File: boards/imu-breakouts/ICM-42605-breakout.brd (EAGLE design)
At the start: 15.2 x 12.7 mm, 5 parts, among them U3 ICM-42605

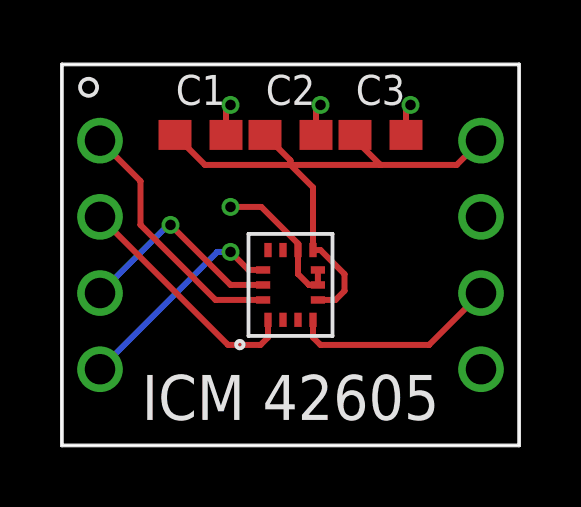
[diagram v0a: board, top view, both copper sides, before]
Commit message: IMU done
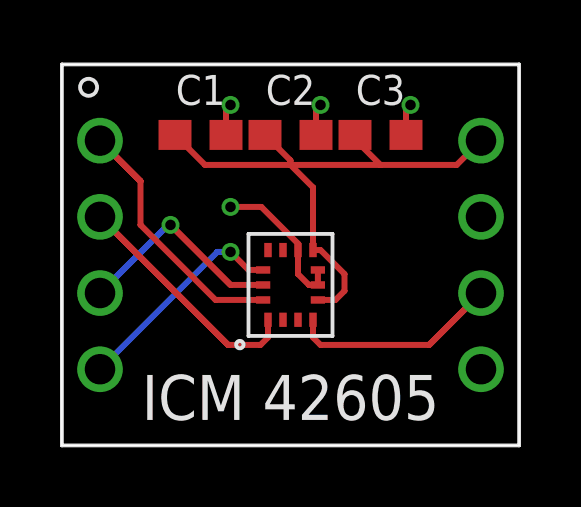
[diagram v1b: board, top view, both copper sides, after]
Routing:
- net MISO: track 8.06 -> 20.1 mm
- net CLK: track 7.21 -> 16.5 mm
- net INT: track 7.01 -> 11.9 mm
- net MOSI: track 8.49 -> 12.3 mm
- net +3.3V: track 19.8 -> 21.8 mm
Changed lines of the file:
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@@
 </layers>
 <board>
-<fusionsync huburn="a.YnVzaW5lc3M6Z2F0ZWNoNzEz" projecturn="a.YnVzaW5lc3M6Z2F0ZWNoNzEzIzIwMjAwNTEwMjk2NDM2NDc2" f3durn="urn:adsk.wipprod:dm.lineage:uCw9H2k5Rae1ZCOXCVSDXA" pcbguid="" lastpulledtime="" lastsyncedchangeguid="" latestrevisionid="f76bd892-a2da-46a4-a104-5053add9c86b" lastsyncedrevisionid="f76bd892-a2da-46a4-a104-5053add9c86b" lastboardhashguid="02177ecb-9c2f-56c7-6b84-e5ea92a8960e" lastpushedtime="2020-05-18T19:52:58Z" linktopcb3d="%12"/>
+<fusionsync huburn="a.YnVzaW5lc3M6Z2F0ZWNoNzEz" projecturn="a.YnVzaW5lc3M6Z2F0ZWNoNzEzIzIwMjAwNTEwMjk2NDM2NDc2" f3durn="urn:adsk.wipprod:dm.lineage:ucu_dVgQRz64XlYRbIqIgQ" pcbguid="" lastpulledtime="" lastsyncedchangeguid="" latestrevisionid="8f9747de-f9ff-40f9-994c-9e28511008a9" lastsyncedrevisionid="8f9747de-f9ff-40f9-994c-9e28511008a9" lastboardhashguid="aa0baad9-2359-efcf-b243-aa71d7df114c" lastpushedtime="2020-05-19T12:59:44Z" linktopcb3d="%12"/>
 <plain>
 <wire x1="-7.62" y1="-6.35" x2="7.62" y2="-6.35" width="0" layer="20"/>
@@
 <text x="0" y="-1" size="1" layer="22" font="vector" ratio="15" rot="MR0" align="bottom-center">IMU
 Breakout v1.0</text>
-<dimension x1="-6.35" y1="3.81" x2="6.35" y2="3.81" x3="0" y3="-1" textsize="1.778" layer="1"/>
+<text x="0" y="2" size="1.5" layer="22" font="vector" ratio="15" rot="MR0" align="bottom-center">2019</text>
 </plain>
 <attributes>
@@
 </autorouter>
 <elements>
-<element name="KIT1" library="RoboJackets-Boards" package="IMU-KIT" value="IMUIMU-KIT" x="0" y="0" smashed="yes"/>
+<element name="KIT1" library="RoboJackets-Boards" package="IMU-KIT" package3d_urn="urn:adsk.eagle:package:20353233/2" override_package3d_urn="urn:adsk.eagle:package:20353233/3" override_package_urn="urn:adsk.eagle:footprint:20353234/1" value="IMUIMU-KIT" x="0" y="0" smashed="yes"/>
 <element name="U3" library="RoboJackets-Sensors" package="ICM-442605-2530091" package3d_urn="urn:adsk.eagle:package:20340429/2" value="ICM-42605" x="0" y="-1" smashed="yes" rot="R90">
 <attribute name="DIGIKEY_LINK" value="https://www.digikey.com/product-detail/en/tdk-invensense/ICM-42605/1428-1152-1-ND/9953675" x="0" y="-1" size="1.778" layer="27" rot="R90" display="off"/>
@@
 <wire x1="1.5" y1="-1.5" x2="1.8" y2="-1.2" width="0.2" layer="1"/>
 <wire x1="1.8" y1="-1.2" x2="1.8" y2="-0.6375" width="0.2" layer="1"/>
+<wire x1="0.75" y1="0.1625" x2="0.75" y2="2.25" width="0.2" layer="1"/>
 </signal>
 <signal name="MOSI">
@@
 <wire x1="-2.5" y1="-1.5" x2="-5" y2="1" width="0.2" layer="1"/>
 <wire x1="-5" y1="1" x2="-5" y2="2.46" width="0.2" layer="1"/>
+<wire x1="-5" y1="2.46" x2="-6.35" y2="3.81" width="0.2" layer="1"/>
+<wire x1="-5" y1="2.46" x2="-6.35" y2="3.81" width="0.2" layer="1"/>
 </signal>
 <signal name="MISO">
@@
 <wire x1="-6.35" y1="1.27" x2="-2.08" y2="-3" width="0.2" layer="1"/>
 <wire x1="-2.08" y1="-3" x2="-1" y2="-3" width="0.2" layer="1"/>
+<wire x1="-6.35" y1="1.27" x2="-2.08" y2="-3" width="0.2" layer="1"/>
+<wire x1="-6.35" y1="1.27" x2="-2.08" y2="-3" width="0.2" layer="1"/>
 </signal>
 <signal name="CLK">
@@
 <wire x1="-2" y1="-1" x2="-4" y2="1" width="0.2" layer="1"/>
 <via x="-4" y="1" extent="1-16" drill="0.35"/>
+<wire x1="-6.35" y1="-1.27" x2="-4.08" y2="1" width="0.2" layer="16"/>
+<wire x1="-2" y1="-1" x2="-4" y2="1" width="0.2" layer="1"/>
+<wire x1="-6.35" y1="-1.27" x2="-4.08" y2="1" width="0.2" layer="16"/>
 </signal>
 <signal name="INT">
@@
 <wire x1="0.75" y1="-2.75" x2="1" y2="-3" width="0.2" layer="1"/>
 <wire x1="1" y1="-3" x2="4.62" y2="-3" width="0.2" layer="1"/>
+<wire x1="4.62" y1="-3" x2="6.35" y2="-1.27" width="0.2" layer="1"/>
+<wire x1="4.62" y1="-3" x2="6.35" y2="-1.27" width="0.2" layer="1"/>
 <wire x1="4.62" y1="-3" x2="6.35" y2="-1.27" width="0.2" layer="1"/>
 </signal>
@@
 packages will not be understood (or retained) with this version.
 </note>
+<note version="9.4" severity="warning">
+Since Version 9.4, EAGLE supports the overriding of 3D packages
+in schematics and board files. Those overridden 3d packages
+will not be understood (or retained) with this version.
+</note>
 </compatibility>
